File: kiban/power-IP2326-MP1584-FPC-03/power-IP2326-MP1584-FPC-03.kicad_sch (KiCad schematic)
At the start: 27 parts, among them J1 BATTERY, J14 CHARGE, J2 BATTERY, J3 BATTERY, J4 DIRECT, J5 LiPo1, J6 LiPo2, J7 VOUT, J8 VIN, J9 OUTPUT, Q2 AO3401A, U1 MAX16054, U2 2S-BMS, U3 IP2326, U5 MP1584EN

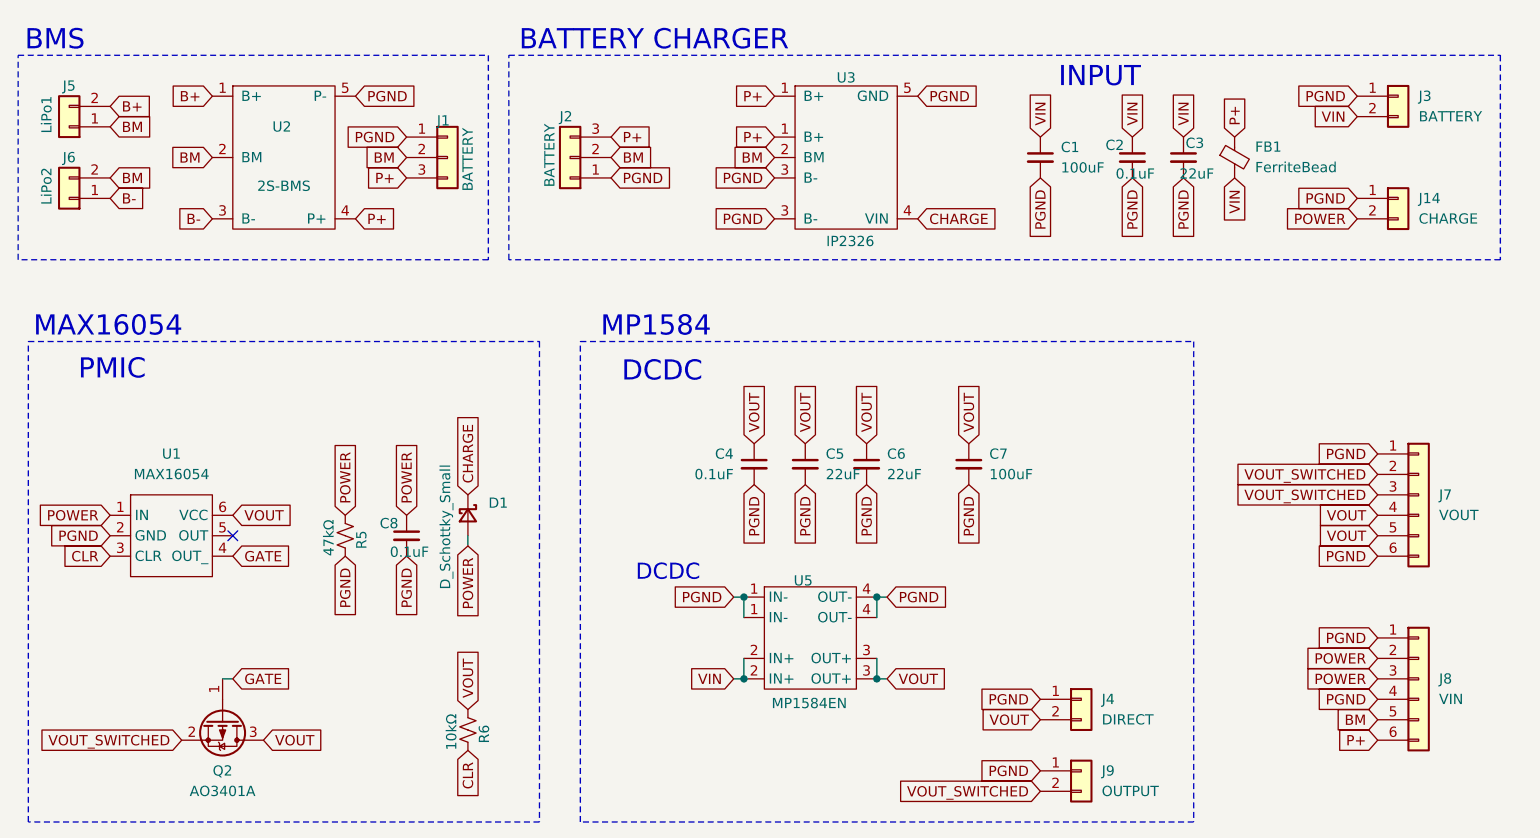
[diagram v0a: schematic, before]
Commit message: kiban: power-IP2326-MP1584-FPC regenerate fab outputs + v02/v03 iterations
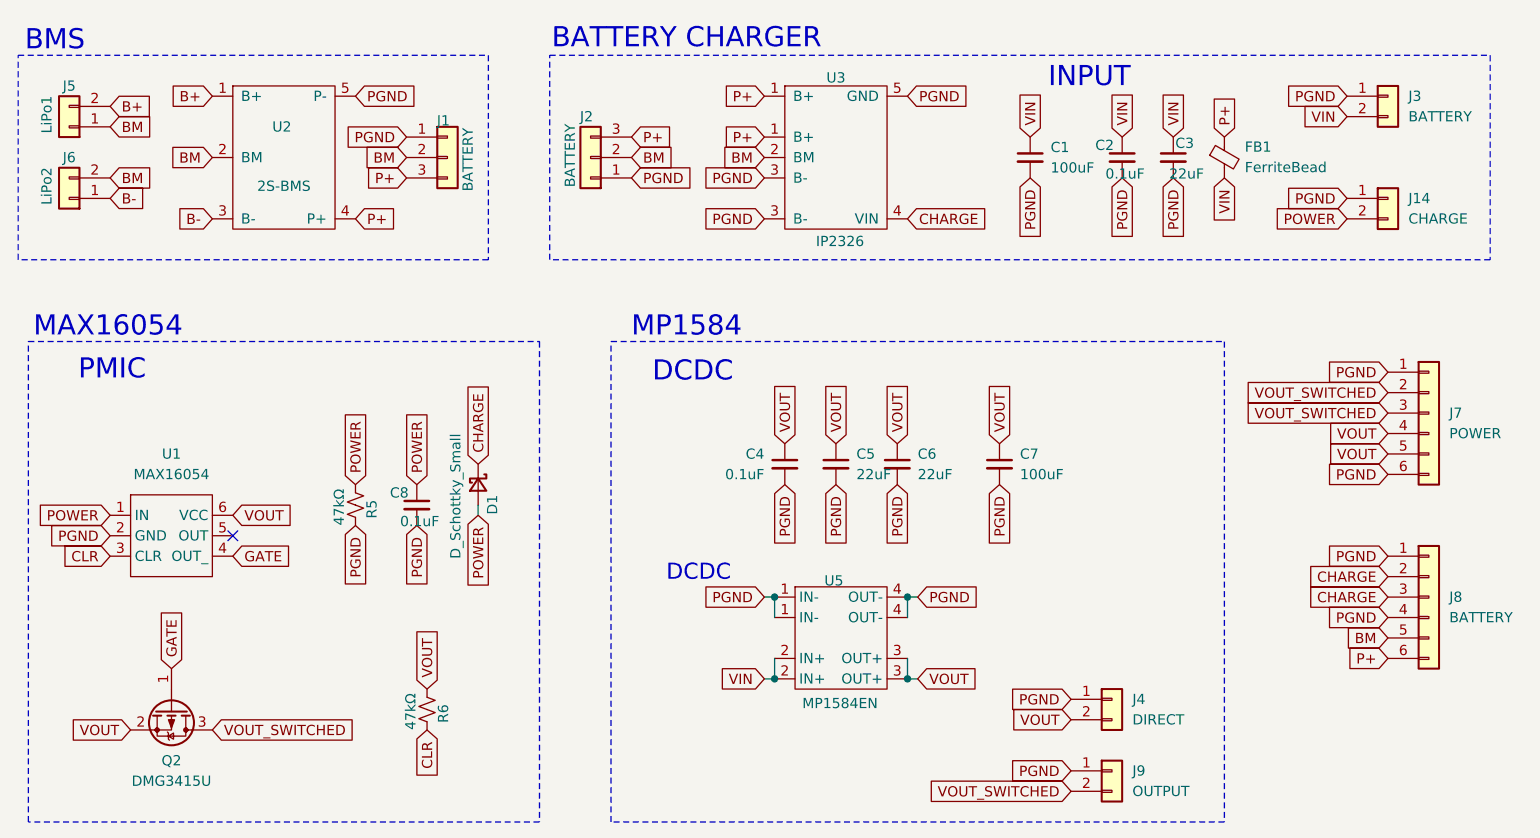
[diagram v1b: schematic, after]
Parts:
- J7: value VOUT -> POWER
- J8: value VIN -> BATTERY
- Q2: value AO3401A -> DMG3415U
- R6: value 10kΩ -> 47kΩ
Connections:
- net CHARGE: now also J8.2 (Pin_2), J8.3 (Pin_3)
- net POWER: no longer J8.2 (Pin_2), J8.3 (Pin_3)
- net VOUT: now also Q2.2 (S); no longer Q2.3 (D)
- net VOUT_SWITCHED: now also Q2.3 (D); no longer Q2.2 (S)
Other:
- moved on the sheet: C1, C2, C3, C4, C5, C6, C7, C8, D1, FB1, J14, J2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
